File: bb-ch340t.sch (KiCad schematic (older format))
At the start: 10 parts, among them U1 CH340H/T, Y1 12.0MHz

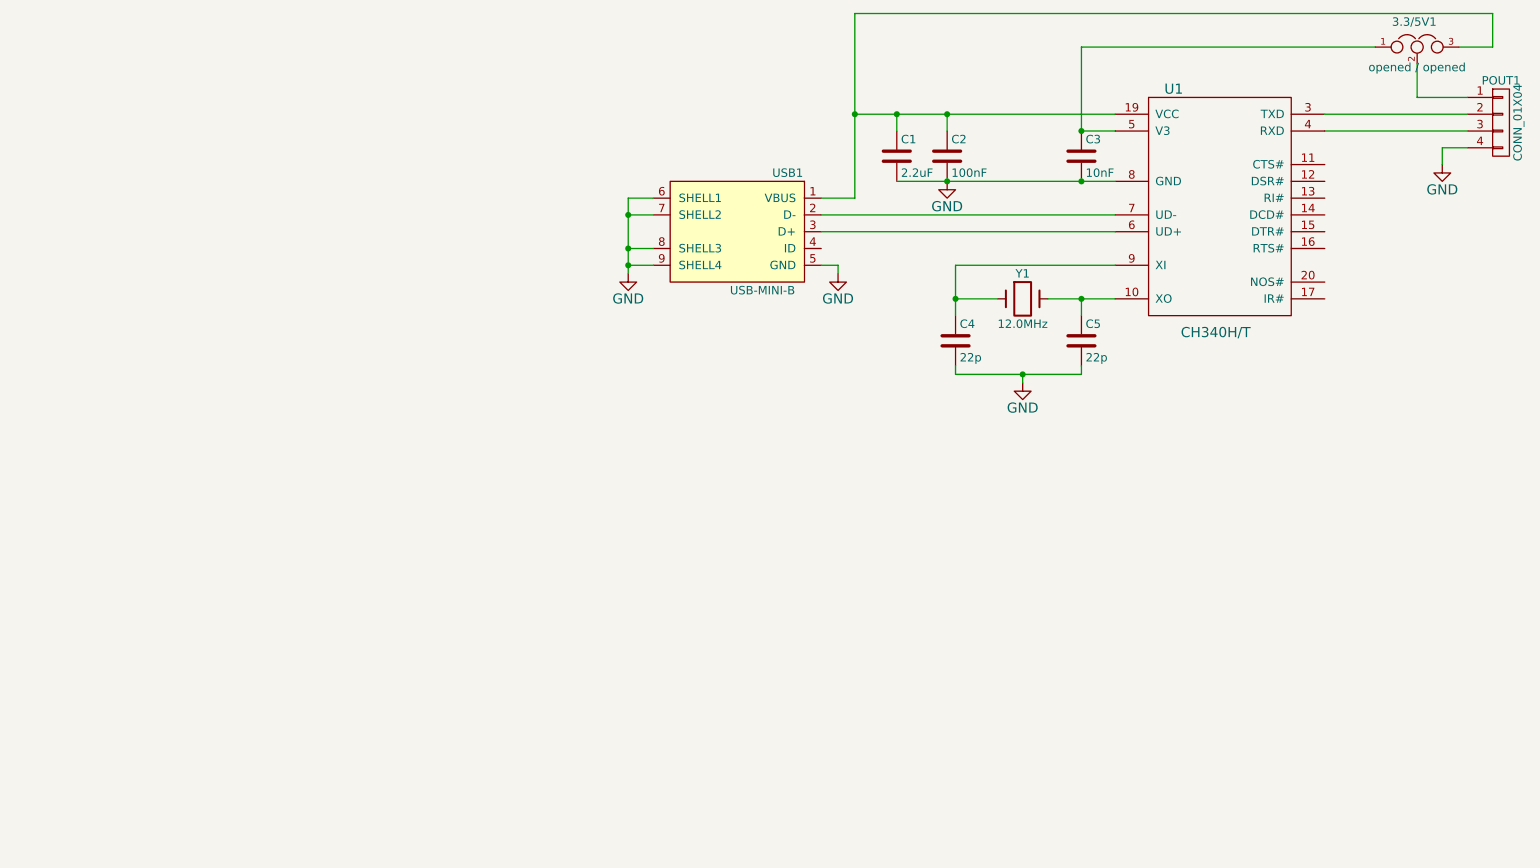
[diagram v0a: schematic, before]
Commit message: Schematic update
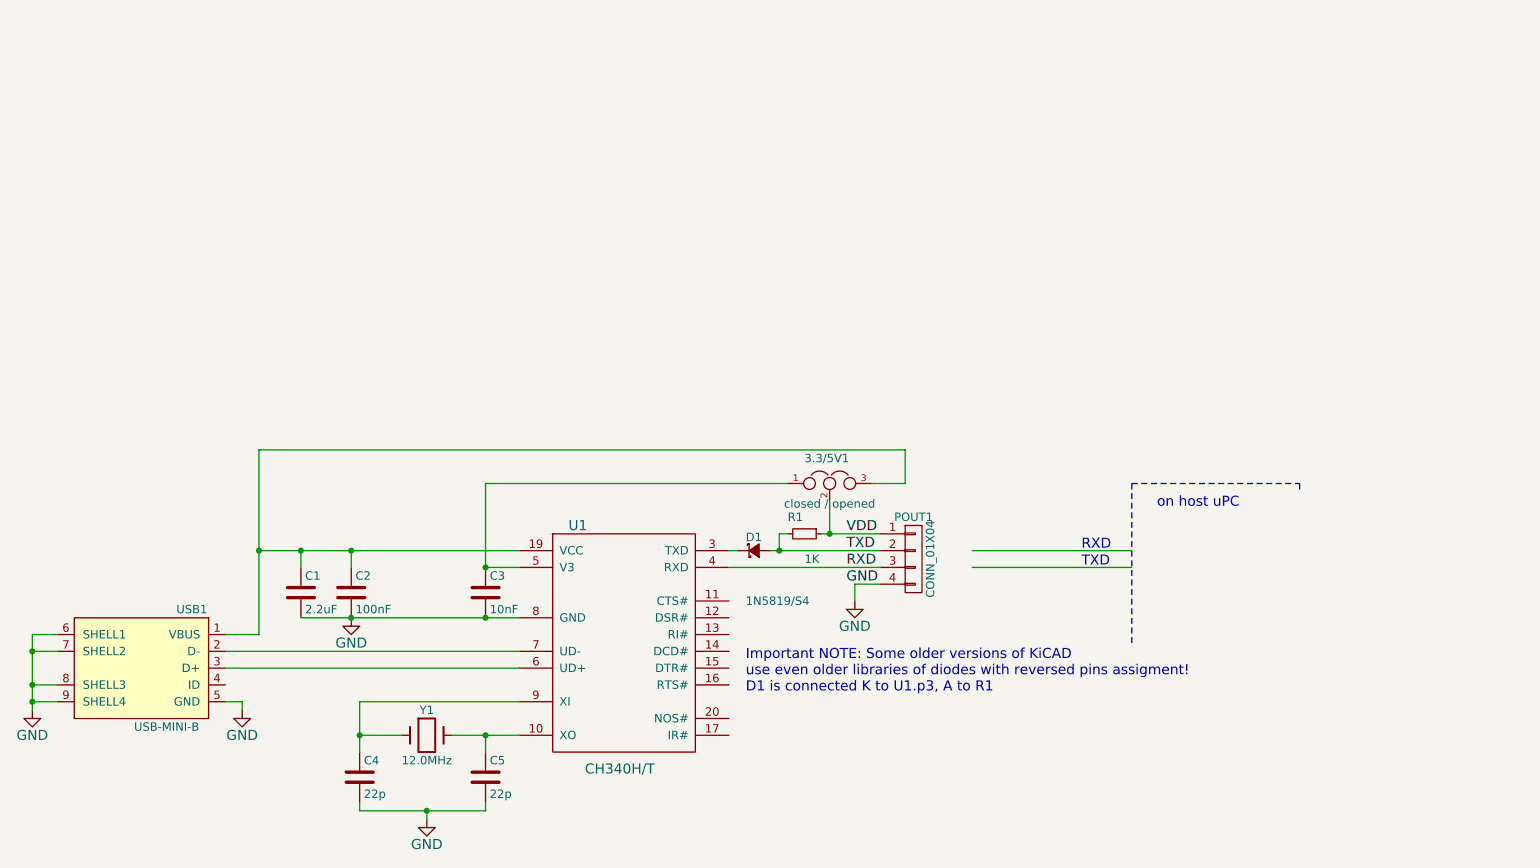
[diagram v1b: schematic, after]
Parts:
- added D1: 1N5819/S4, symbol D_Schottky_Small
- added R1: 1K, symbol R_Small
- 3.3/5V1: value opened / opened -> closed / opened
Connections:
- net labels added: RXD, TXD, VDD
- wire segments 36 -> 41
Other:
- note added: "Important NOTE: Some older versions of KiCAD\nuse even older libraries of diodes with reversed pins assigment!\nD1 is connected K to U1.p3, A to R1"
- note added: "RXD"
- note added: "TXD"
- note added: "on host uPC"
- moved on the sheet: 3.3/5V1, C1, C2, C3, C4, C5, POUT1, U1, USB1, Y1
